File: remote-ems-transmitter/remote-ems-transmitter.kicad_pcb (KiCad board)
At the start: 2 copper layers, 65 x 30 mm, 59 parts, among them IC1 Wio-E5, J1 Conn_01x04_Pin, J2 Conn_01x02, J3 Conn_01x02, J4 Conn_Coaxial, J5 USB_C_Receptacle_USB2.0, J6 Conn_01x02_Pin, Q1 BSS138, SW1 SW_Push, SW2 SW_Push, SW3 SW_Push, SW4 2MS1-T2-B4-VS2-Q-E-S, U1 STM32G431K8Tx, U2 MCP73831-2-OT, U3 NJM12888F33, U4 XC8111AA01MR-G, U5 XC8111AA01MR-G

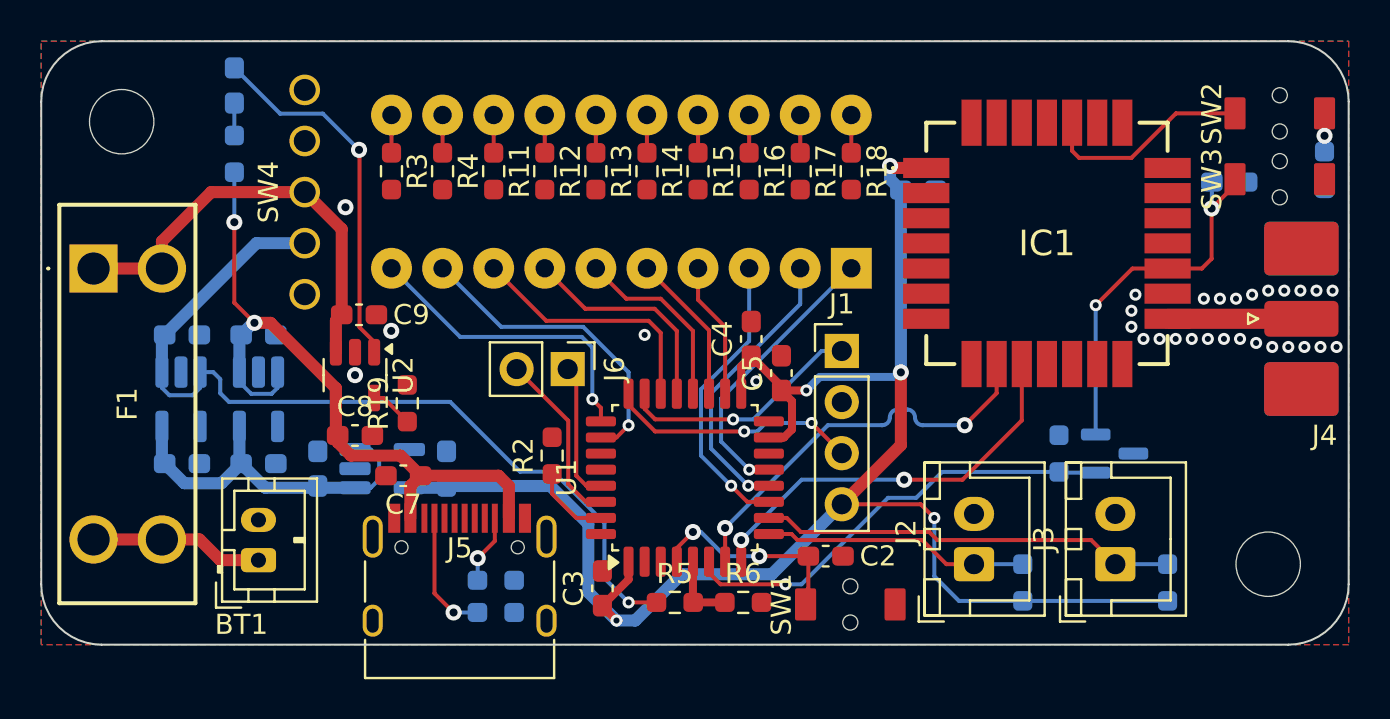
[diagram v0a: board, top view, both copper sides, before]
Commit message: LED周り修正
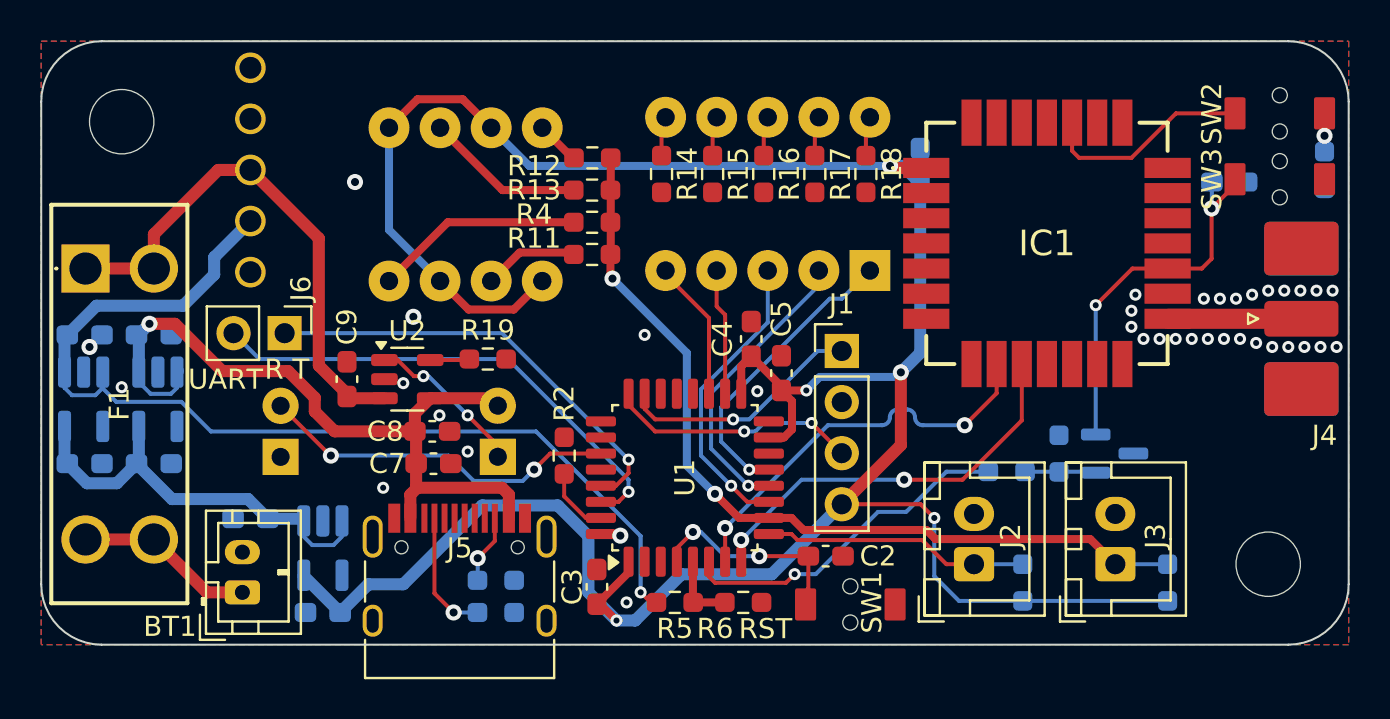
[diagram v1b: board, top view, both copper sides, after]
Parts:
- removed R21: 1k, Resistor_SMD:R_0603_1608Metric_Pad0.98x0.95mm_HandSolder
- added BAR2: OSX40601-AO, 0Ikedalibrary:OSX40601-AO, B.Cu at (36.1, 23.1)
- added D2: LED, LED_THT:LED_D5.0mm_FlatTop, B.Cu at (26.9, 35.7)
- BAR1: value HDSP-4830_2 -> OSX05201-GGR1; footprint Display:HDSP-4830 -> 0Ikedalibrary:OSX05201-GGR1
- D1: footprint LED_SMD:LED_0603_1608Metric_Pad1.05x0.95mm_HandSolder -> LED_THT:LED_D5.0mm_FlatTop
- R3: value 4.7k -> 100; moved to B.Cu
- SW4: moved to B.Cu
- moved R3 34.0 mm to (63.0, 36.4), turned to 0 degrees
- moved D1 22.6 mm to (37.7, 35.7), turned to 90 degrees
- moved J6 14.2 mm to (27.1, 29.5)
- moved BAR1 11.7 mm to (44.2, 22.4)
- moved C11 9.43 mm to (29.0, 43.4), turned to 180 degrees
- moved R4 7.85 mm to (42.4, 24.0), turned to 0 degrees
- moved R11 6.41 mm to (42.4, 25.6), turned to 0 degrees
- moved C14 5.20 mm to (20.6, 29.6)
- moved C15 5.20 mm to (20.6, 36.0)
- moved U5 5.00 mm to (20.8, 32.8)
- moved U3 4.93 mm to (29.0, 40.2), turned to -90 degrees
- moved C12 4.84 mm to (17.2, 29.6)
- moved C13 4.84 mm to (17.2, 36.0)
- moved U4 4.84 mm to (17.1, 32.8)
- moved R19 4.57 mm to (37.2, 30.8), turned to 0 degrees
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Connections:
- BAR1 pad 10: LED_opt_supply9 -> Net-(BAR1-K-Pad10)
- BAR1 pad 6: LED_opt_supply5 -> Net-(BAR1-K-Pad6)
- BAR1 pad 7: LED_opt_supply6 -> Net-(BAR1-K-Pad7)
- BAR1 pad 8: LED_opt_supply7 -> Net-(BAR1-K-Pad8)
- BAR1 pad 9: LED_opt_supply8 -> Net-(BAR1-K-Pad9)
- D1 pad 2: Net-(D1-A) -> VBUS
- Q1 pad 1: Wio-RST -> Net-(Q1-G)
- R11 pad 1: Net-(BAR1-K-Pad13) -> Net-(BAR2-K-Pad6)
- R11 pad 2: GNDD -> SW
- R12 pad 1: Net-(BAR1-K-Pad14) -> Net-(BAR2-A-Pad4)
- R12 pad 2: GNDD -> SW
- R13 pad 1: Net-(BAR1-K-Pad15) -> Net-(BAR2-A-Pad2)
- R13 pad 2: GNDD -> SW
- R14 pad 1: Net-(BAR1-K-Pad16) -> Net-(BAR1-K-Pad6)
- R15 pad 1: Net-(BAR1-K-Pad17) -> Net-(BAR1-K-Pad7)
- R16 pad 1: Net-(BAR1-K-Pad18) -> Net-(BAR1-K-Pad8)
- R17 pad 1: Net-(BAR1-K-Pad19) -> Net-(BAR1-K-Pad9)
- R18 pad 1: Net-(BAR1-K-Pad20) -> Net-(BAR1-K-Pad10)
- R3 pad 1: Net-(BAR1-K-Pad11) -> Wio-RST
- R3 pad 2: GNDD -> Net-(Q1-G)
- R4 pad 1: Net-(BAR1-K-Pad12) -> Net-(BAR2-K-Pad8)
- R4 pad 2: GNDD -> SW
- R8 pad 1: Wio-RST -> Net-(Q1-G)
- U1 pad 20: LED_opt_supply5 -> unconnected-(U1-PA10-Pad20)
- U1 pad 21: LED_opt_supply6 -> unconnected-(U1-PA11-Pad21)
- U1 pad 22: LED_opt_supply7 -> unconnected-(U1-PA12-Pad22)
- U1 pad 25: LED_opt_supply9 -> unconnected-(U1-PA15-Pad25)
- U1 pad 26: LED_opt_supply8 -> unconnected-(U1-PB3-Pad26)
- U1 pad 28: LED2 -> unconnected-(U1-PB5-Pad28)
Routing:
- net +3.3V: track 86.6 -> 137.3 mm
- net SW: track 20.8 -> 42.8 mm, vias 0 -> 2
- net LED1: track 0.00 -> 18.0 mm, vias 0 -> 2
- net UART_RX: track 8.77 -> 24.8 mm, vias 0 -> 1
- net LED_opt_supply8: track 15.7 -> 0.00 mm, vias 1 -> 0
- net LED_opt_supply9: track 15.5 -> 0.00 mm, vias 1 -> 0
- net UART_TX: track 6.91 -> 22.0 mm, vias 0 -> 1
- net LED_opt_supply7: track 12.7 -> 0.00 mm
- net LED_opt_supply6: track 11.0 -> 0.00 mm
- net Net-(BAR2-K-Pad8): track 0.00 -> 10.4 mm
- net STAT: track 18.3 -> 7.96 mm, vias 1 -> 2
- net LED_opt_supply5: track 9.24 -> 0.00 mm
- net +BATT: track 44.0 -> 52.0 mm
- net Net-(BAR2-A-Pad2): track 0.00 -> 7.93 mm
- net Wio-RST: track 22.3 -> 16.8 mm
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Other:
- board text added: "R T"
- board text added: "RST"
- board text added: "UART"
